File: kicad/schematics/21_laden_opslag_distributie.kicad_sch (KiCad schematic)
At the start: 4 parts

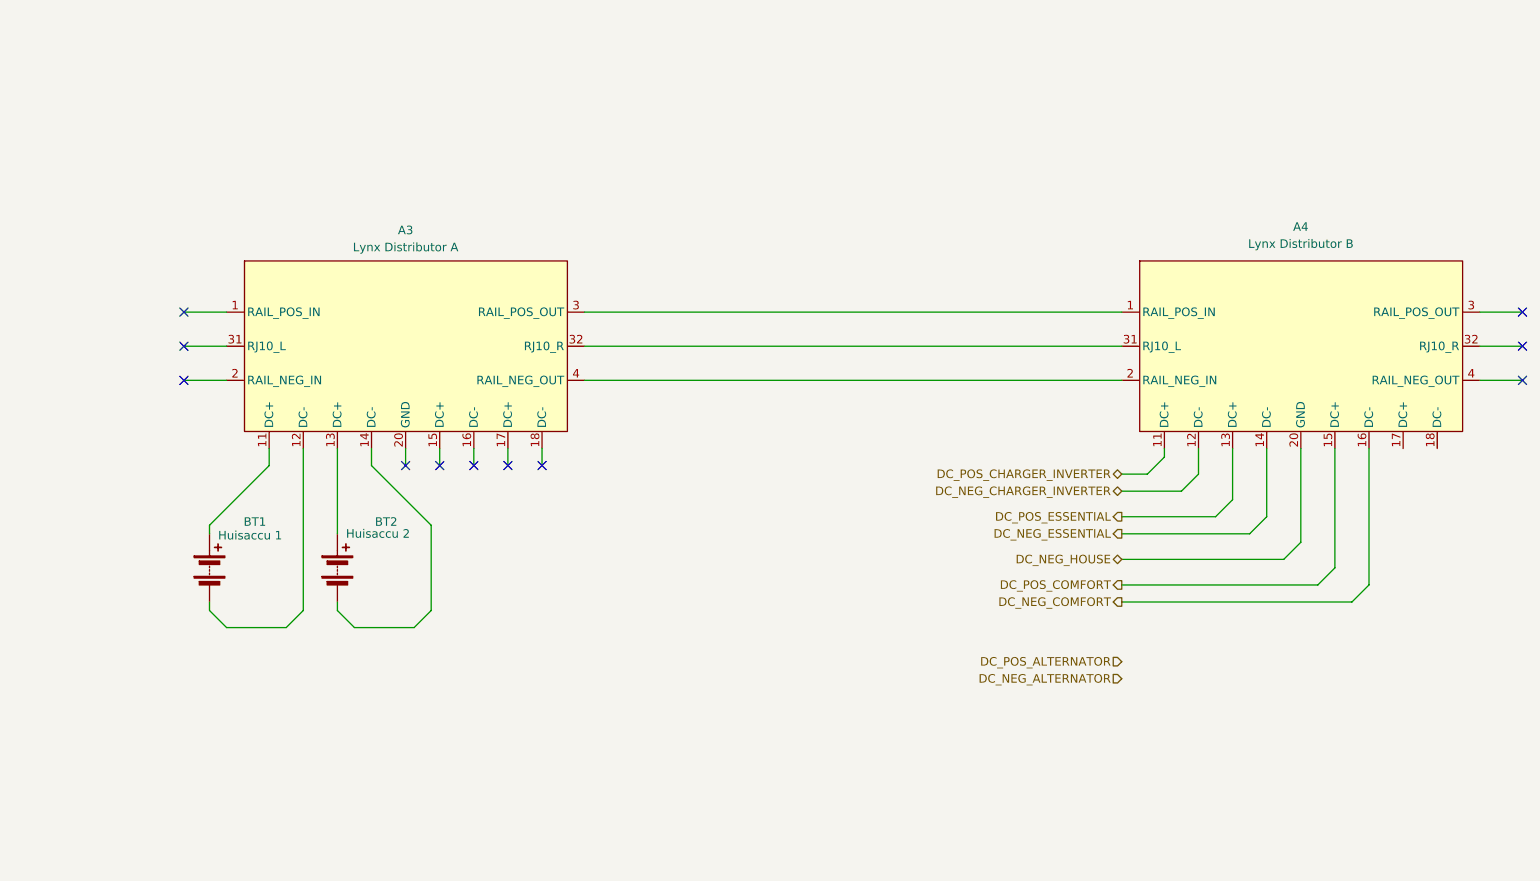
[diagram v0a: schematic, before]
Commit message: Vervolg 21_laden_opslag_distributie
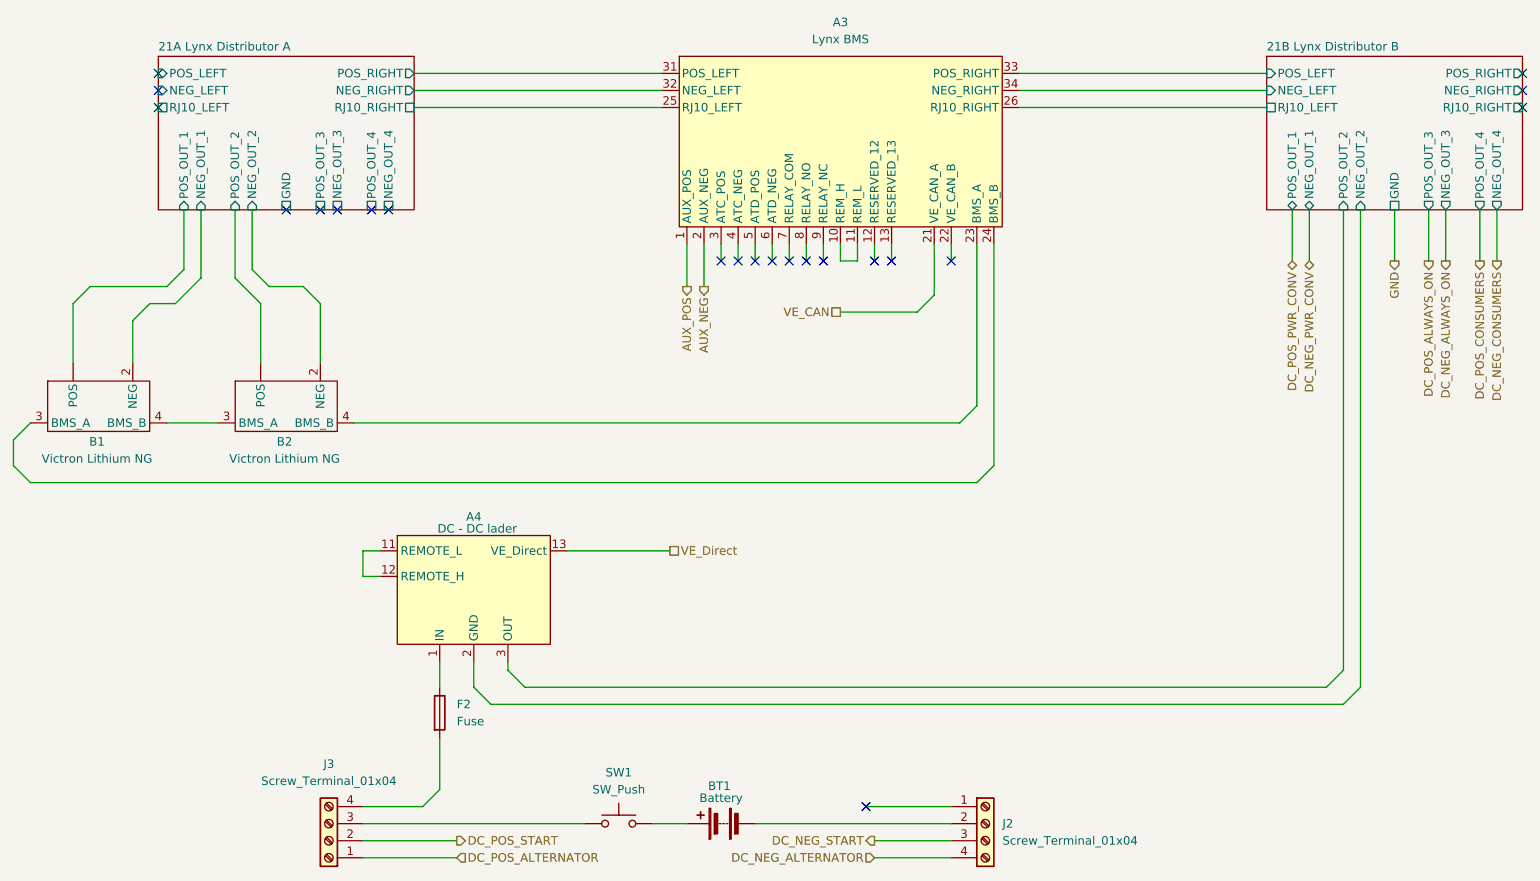
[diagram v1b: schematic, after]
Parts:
- removed A3: Lynx Distributor A, symbol falkor-electrical:lynx_distributor
- removed A4: Lynx Distributor B, symbol falkor-electrical:lynx_distributor
- removed BT2: Huisaccu 2, symbol Device:Battery
- added A3: Lynx BMS, symbol falkor-electrical:lynx_bms
- added A4: DC - DC lader, symbol falkor-electrical:Orion_XS
- added B1, B2: Victron Lithium NG, symbol falkor-electrical:Victron_NG_Accu
- added F2: Fuse, symbol Device:Fuse
- added J2, J3: Screw_Terminal_01x04, symbol Connector:Screw_Terminal_01x04
- added SW1: SW_Push, symbol Switch:SW_Push
- BT1: value Huisaccu 1 -> Battery
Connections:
- net DC_NEG_ALTERNATOR: now also J2.4 (Pin_4)
- net DC_POS_ALTERNATOR: now also J3.1 (Pin_1)
- net at BT1.1 (+): now also SW1.2
- net at BT1.2 (-): now also J2.2 (Pin_2)
- new net: B1.4 (BMS_B), B2.3 (BMS_A)
- new net: A3.23 (BMS_A), B2.4 (BMS_B)
- new net: J3.3 (Pin_3), SW1.1
- new net: F2.2, J3.4 (Pin_4)
- new net: A4.1 (IN), F2.1
- new net: A4.11 (REMOTE_L), A4.12 (REMOTE_H)
- new net: A3.10 (REM_H), A3.11 (REM_L)
- new net: A3.24 (BMS_B), B1.3 (BMS_A)
- new net 21A Lynx Distributor A/NEG_OUT_1: B1.2 (NEG)
- new net 21A Lynx Distributor A/NEG_OUT_2: B2.2 (NEG)
- new net 21A Lynx Distributor A/NEG_RIGHT: A3.32 (NEG_LEFT)
- new net 21A Lynx Distributor A/POS_OUT_1: B1. (POS)
- new net 21A Lynx Distributor A/POS_OUT_2: B2. (POS)
- new net 21A Lynx Distributor A/POS_RIGHT: A3.31 (POS_LEFT)
- new net 21A Lynx Distributor A/RJ10_RIGHT: A3.25 (RJ10_LEFT)
- new net 21B Lynx Distributor B/NEG_LEFT: A3.34 (NEG_RIGHT)
- new net 21B Lynx Distributor B/NEG_OUT_2: A4.2 (GND)
- new net 21B Lynx Distributor B/POS_LEFT: A3.33 (POS_RIGHT)
- new net 21B Lynx Distributor B/POS_OUT_2: A4.3 (OUT)
- new net 21B Lynx Distributor B/RJ10_LEFT: A3.26 (RJ10_RIGHT)
- new net AUX_NEG: A3.2 (AUX_NEG)
- new net AUX_POS: A3.1 (AUX_POS)
- new net DC_NEG_START: J2.3 (Pin_3)
- new net DC_POS_START: J3.2 (Pin_2)
- new net VE_CAN: A3.21 (VE_CAN_A)
- new net VE_Direct: A4.13 (VE_Direct)
- no-connect marks 11 -> 22
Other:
- added sheet 21A Lynx Distributor A (21a_lynx_distributor_a.kicad_sch)
- added sheet 21B Lynx Distributor B (21a_lynx_distributor_a.kicad_sch)
- moved on the sheet: BT1
